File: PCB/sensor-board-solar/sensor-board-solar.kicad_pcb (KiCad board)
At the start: 2 copper layers, 23.6 x 23.5 mm, 7 parts, among them J1 Conn_01x02_Pin (Solar panel c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, U1 MAGNETIC POGO CONN., U2 MAGNETIC POGO CONN.

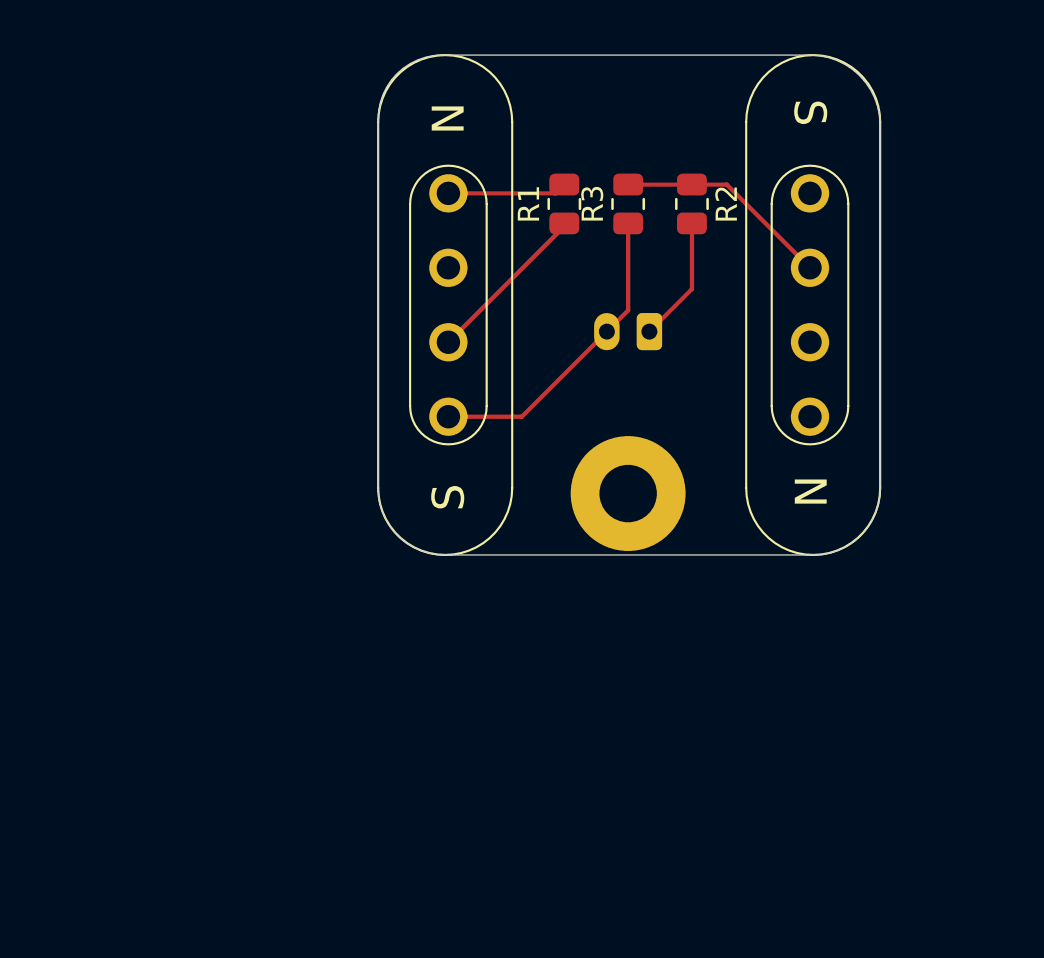
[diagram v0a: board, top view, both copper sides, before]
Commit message: Update PCB files (pressure + solar)#
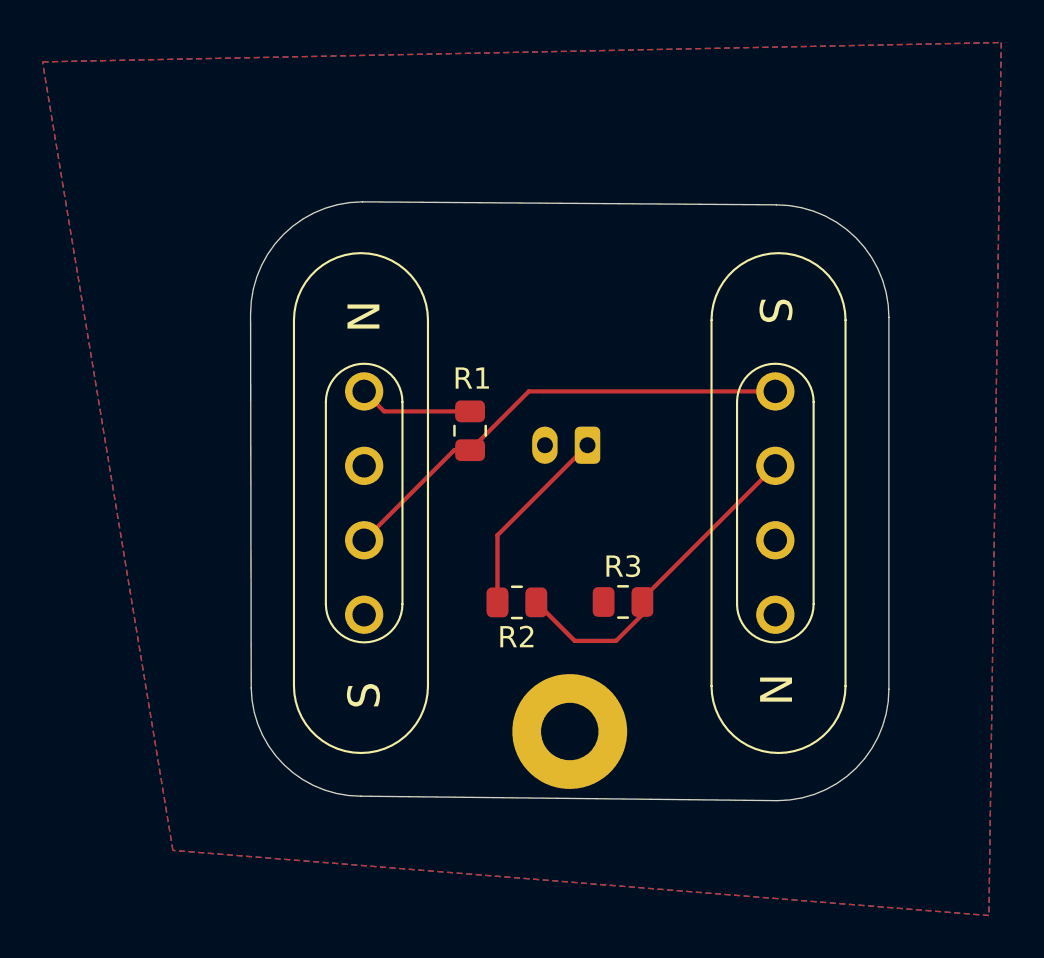
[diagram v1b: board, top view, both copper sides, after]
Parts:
- added G***: LOGO, LOGO, B.Cu at (137.7, 97.2)
- moved R2 20.5 mm to (135.2, 97.7), turned to 180 degrees
- moved R3 18.7 mm to (140.2, 97.7), turned to 0 degrees
- moved R1 11.5 mm to (133.0, 89.7)
- moved H1 11.5 mm to (137.7, 103.8)
- moved U2 10.1 mm to (128.0, 93.1)
- moved U1 9.45 mm to (147.4, 93.1)
- moved J1 6.08 mm to (138.5, 90.3)
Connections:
- U1 pad 1: unconnected-(U1-Pad1) -> +3.3V
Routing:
- net +3.3V: track 7.84 -> 22.7 mm
- net GND: track 14.6 -> 0.00 mm
- net /ADC: track 10.2 -> 15.8 mm
- net Net-(J1-Pin_1): track 5.92 -> 9.14 mm
- added copper zone on B.Cu, net GND
- added copper zone on F.Cu, net GND
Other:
- board size 23.6 x 23.5 mm -> 30 x 28.1 mm
- board text added: "BOREALIS"
- board text added: "VOLTMETER"
- board text removed: "Borealis Voltmeter"
